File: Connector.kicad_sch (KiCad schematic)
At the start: 5 parts, among them J6 Conn_02x10_Odd_Even

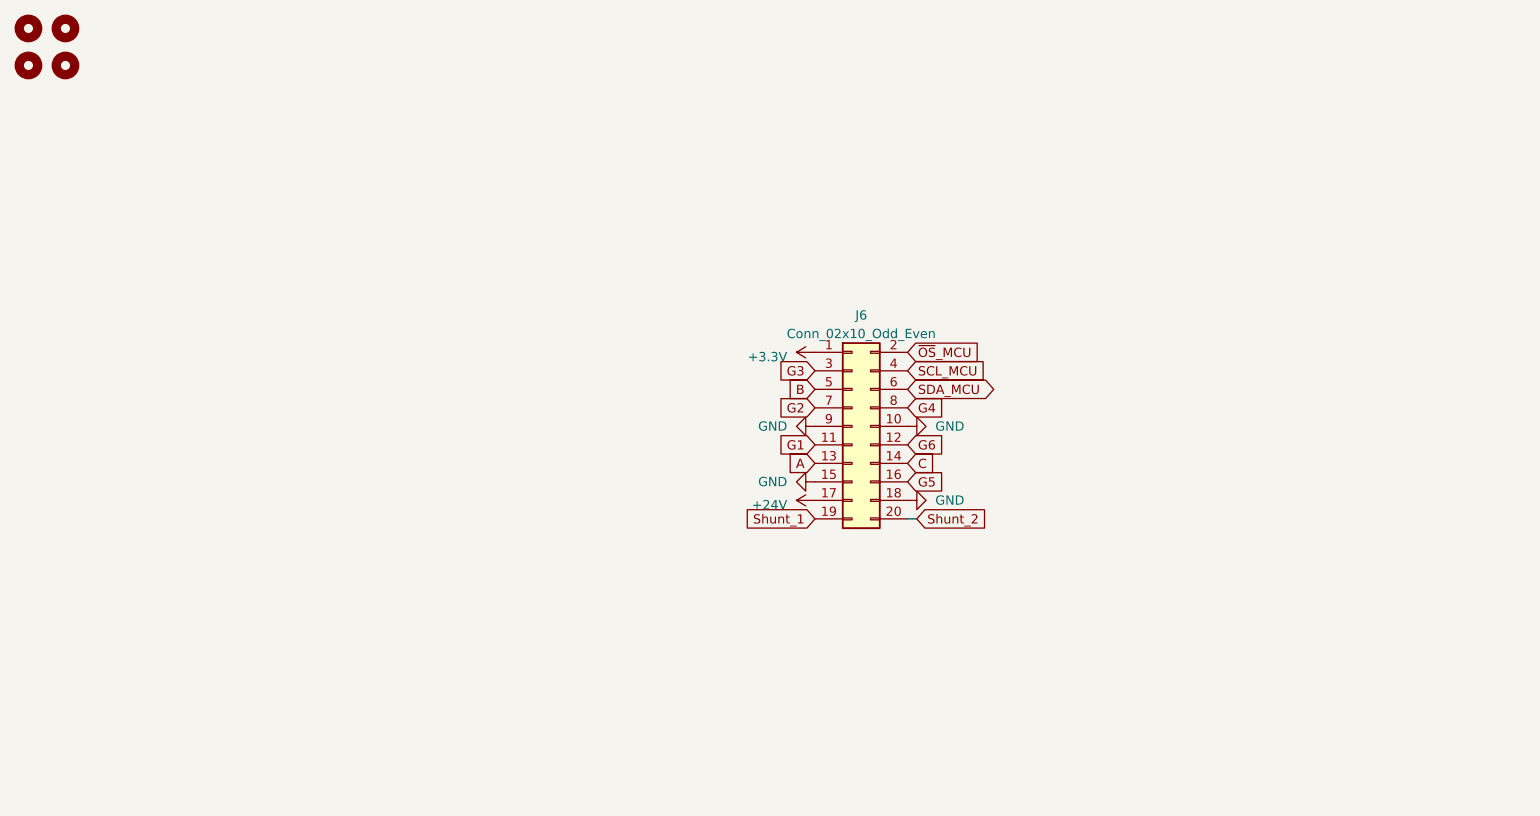
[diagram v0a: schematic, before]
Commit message: Отчётная версия
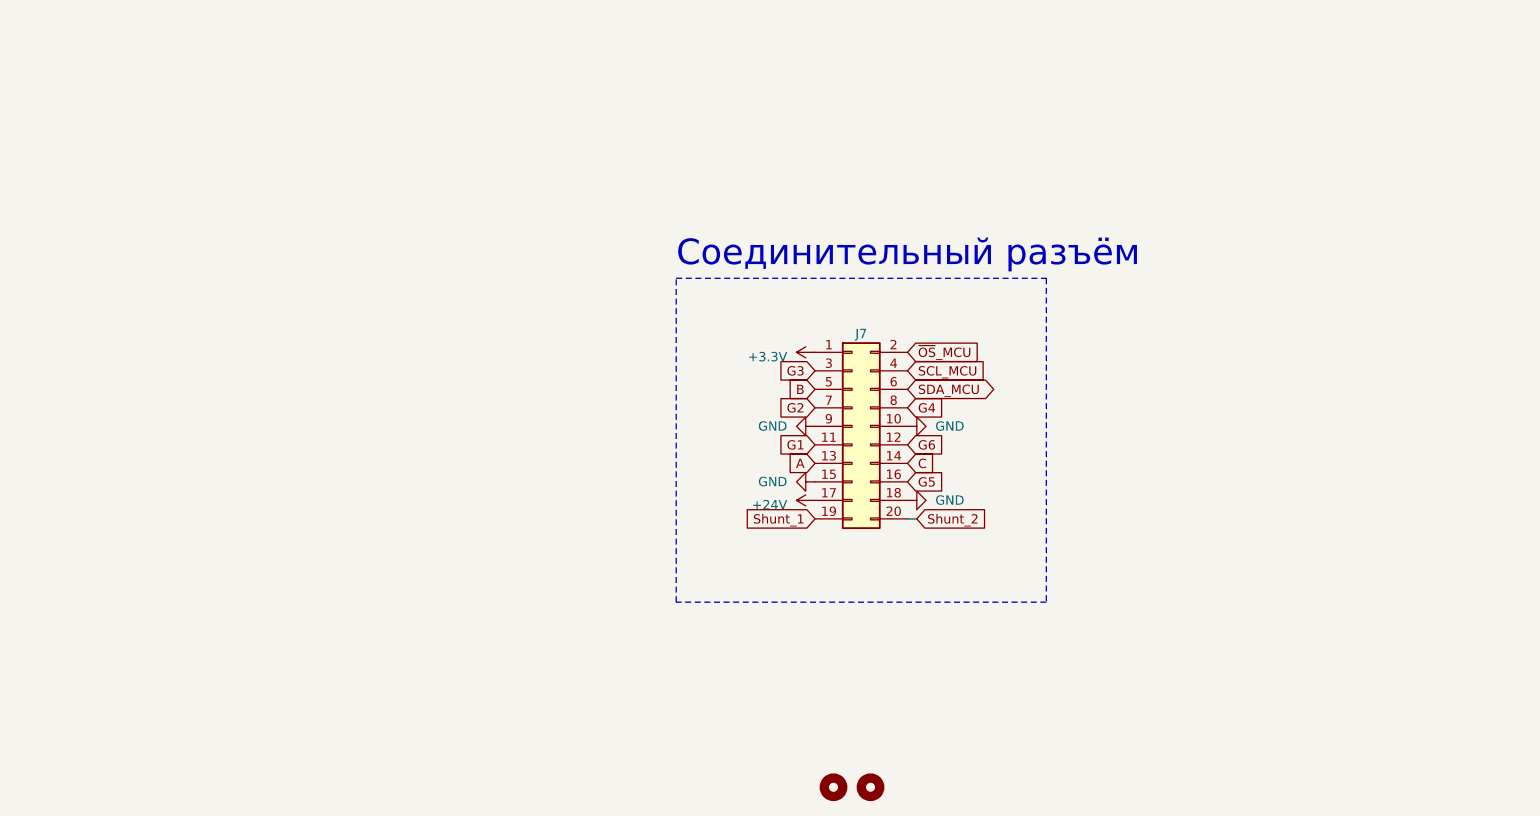
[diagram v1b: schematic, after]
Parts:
- removed H3, H4: MountingHole, MountingHole:MountingHole_3.2mm_M3, symbol Mechanical:MountingHole
- renumbered J6 to J7
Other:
- note added: "Соединительный разъём"
- company: (none) -> Московский Политех
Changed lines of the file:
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@@
 (kicad_sch (version 20230121) (generator eeschema)
   (paper "A4")
+  (title_block
+    (company "Московский Политех")
+    (comment 1 "МПСТ.76721.758764.01.Э3.М")
+  )
   (wire (pts (xy 163.83 96.52) (xy 165.1 96.52))
     (stroke (width 0) (type default))
   )
+  (rectangle (start 132.08 63.5) (end 182.88 107.95)
+    (stroke (width 0) (type dash))
+    (fill (type none))
+  )
+  (text "Соединительный разъём" (at 132.08 62.23 0)
+    (effects (font (size 3.5 3.5)) (justify left bottom))
+  )
   (global_label "C" (shape input) (at 163.83 88.9 0) (fields_autoplaced)
     (effects (font (size 1.27 1.27)) (justify left))
@@
   (symbol (lib_id "power:GND") (at 151.13 91.44 270) (unit 1)
     (in_bom yes) (on_board yes) (dnp no) (fields_autoplaced)
-    (property "Reference" "#PWR018" (at 144.78 91.44 0)
+    (property "Reference" "#PWR019" (at 144.78 91.44 0)
       (effects (font (size 1.27 1.27)) hide)
     )
@@
       (project "Силовая плата"
         (path "/96c6fc92-8ec6-44f7-b0dc-9ad8f1acea09/a27b443f-c036-4fd6-934c-6ea912709de0"
-          (reference "#PWR018") (unit 1)
+          (reference "#PWR019") (unit 1)
+        )
+        (path "/96c6fc92-8ec6-44f7-b0dc-9ad8f1acea09/e8223907-1cc2-45fb-8266-c61760002ef3"
+          (reference "#PWR038") (unit 1)
         )
       )
@@
   )
   (symbol (lib_id "Connector_Generic:Conn_02x10_Odd_Even") (at 156.21 83.82 0) (unit 1)
-    (in_bom yes) (on_board yes) (dnp no) (fields_autoplaced)
-    (property "Reference" "J6" (at 157.48 68.58 0)
+    (in_bom yes) (on_board yes) (dnp no)
+    (property "Reference" "J7" (at 157.48 71.12 0)
       (effects (font (size 1.27 1.27)))
     )
     (property "Value" "Conn_02x10_Odd_Even" (at 157.48 71.12 0)
-      (effects (font (size 1.27 1.27)))
+      (effects (font (size 1.27 1.27)) hide)
     )
     (property "Footprint" "Connector_PinSocket_2.54mm:PinSocket_2x10_P2.54mm_Vertical" (at 156.21 83.82 0)
@@
       (project "Силовая плата"
         (path "/96c6fc92-8ec6-44f7-b0dc-9ad8f1acea09/a27b443f-c036-4fd6-934c-6ea912709de0"
-          (reference "J6") (unit 1)
-        )
-      )
-    )
-  )
-  (symbol (lib_id "Mechanical:MountingHole") (at 48.26 34.29 0) (unit 1)
-    (in_bom yes) (on_board yes) (dnp no) (fields_autoplaced)
-    (property "Reference" "H4" (at 50.8 33.655 0)
-      (effects (font (size 1.27 1.27)) (justify left) hide)
-    )
-    (property "Value" "MountingHole" (at 50.8 36.195 0)
-      (effects (font (size 1.27 1.27)) (justify left) hide)
-    )
-    (property "Footprint" "MountingHole:MountingHole_3.2mm_M3" (at 48.26 34.29 0)
-      (effects (font (size 1.27 1.27)) hide)
-    )
-    (property "Datasheet" "~" (at 48.26 34.29 0)
-      (effects (font (size 1.27 1.27)) hide)
-    )
-    (instances
-      (project "Силовая плата"
-        (path "/96c6fc92-8ec6-44f7-b0dc-9ad8f1acea09/a27b443f-c036-4fd6-934c-6ea912709de0"
-          (reference "H4") (unit 1)
-        )
-      )
-    )
-  )
-  (symbol (lib_id "Mechanical:MountingHole") (at 43.18 34.29 0) (unit 1)
-    (in_bom yes) (on_board yes) (dnp no) (fields_autoplaced)
-    (property "Reference" "H3" (at 45.72 33.655 0)
-      (effects (font (size 1.27 1.27)) (justify left) hide)
-    )
-    (property "Value" "MountingHole" (at 45.72 36.195 0)
-      (effects (font (size 1.27 1.27)) (justify left) hide)
-    )
-    (property "Footprint" "MountingHole:MountingHole_3.2mm_M3" (at 43.18 34.29 0)
-      (effects (font (size 1.27 1.27)) hide)
-    )
-    (property "Datasheet" "~" (at 43.18 34.29 0)
-      (effects (font (size 1.27 1.27)) hide)
-    )
-    (instances
-      (project "Силовая плата"
-        (path "/96c6fc92-8ec6-44f7-b0dc-9ad8f1acea09/a27b443f-c036-4fd6-934c-6ea912709de0"
-          (reference "H3") (unit 1)
+          (reference "J7") (unit 1)
+        )
+        (path "/96c6fc92-8ec6-44f7-b0dc-9ad8f1acea09/e8223907-1cc2-45fb-8266-c61760002ef3"
+          (reference "J9") (unit 1)
         )
       )
@@
         )
         (path "/96c6fc92-8ec6-44f7-b0dc-9ad8f1acea09/a27b443f-c036-4fd6-934c-6ea912709de0"
-          (reference "#PWR023") (unit 1)
+          (reference "#PWR020") (unit 1)
+        )
+        (path "/96c6fc92-8ec6-44f7-b0dc-9ad8f1acea09/e8223907-1cc2-45fb-8266-c61760002ef3"
+          (reference "#PWR039") (unit 1)
         )
       )
@@
   (symbol (lib_id "power:+3.3V") (at 151.13 73.66 90) (unit 1)
     (in_bom yes) (on_board yes) (dnp no) (fields_autoplaced)
-    (property "Reference" "#PWR042" (at 154.94 73.66 0)
+    (property "Reference" "#PWR016" (at 154.94 73.66 0)
       (effects (font (size 1.27 1.27)) hide)
     )
@@
       (project "Силовая плата"
         (path "/96c6fc92-8ec6-44f7-b0dc-9ad8f1acea09/a27b443f-c036-4fd6-934c-6ea912709de0"
-          (reference "#PWR042") (unit 1)
-        )
-      )
-    )
-  )
-  (symbol (lib_id "Mechanical:MountingHole") (at 48.26 29.21 0) (unit 1)
-    (in_bom yes) (on_board yes) (dnp no) (fields_autoplaced)
-    (property "Reference" "H2" (at 50.8 28.575 0)
-      (effects (font (size 1.27 1.27)) (justify left) hide)
-    )
-    (property "Value" "MountingHole" (at 50.8 31.115 0)
-      (effects (font (size 1.27 1.27)) (justify left) hide)
-    )
-    (property "Footprint" "MountingHole:MountingHole_3.2mm_M3" (at 48.26 29.21 0)
-      (effects (font (size 1.27 1.27)) hide)
-    )
-    (property "Datasheet" "~" (at 48.26 29.21 0)
+          (reference "#PWR016") (unit 1)
+        )
+        (path "/96c6fc92-8ec6-44f7-b0dc-9ad8f1acea09/e8223907-1cc2-45fb-8266-c61760002ef3"
+          (reference "#PWR035") (unit 1)
+        )
+      )
+    )
+  )
+  (symbol (lib_id "Mechanical:MountingHole") (at 158.75 133.35 0) (unit 1)
+    (in_bom yes) (on_board yes) (dnp no) (fields_autoplaced)
+    (property "Reference" "H2" (at 161.29 132.715 0)
+      (effects (font (size 1.27 1.27)) (justify left) hide)
+    )
+    (property "Value" "MountingHole" (at 161.29 135.255 0)
+      (effects (font (size 1.27 1.27)) (justify left) hide)
+    )
+    (property "Footprint" "MountingHole:MountingHole_3.2mm_M3" (at 158.75 133.35 0)
+      (effects (font (size 1.27 1.27)) hide)
+    )
+    (property "Datasheet" "~" (at 158.75 133.35 0)
       (effects (font (size 1.27 1.27)) hide)
     )
@@
         (path "/96c6fc92-8ec6-44f7-b0dc-9ad8f1acea09/a27b443f-c036-4fd6-934c-6ea912709de0"
           (reference "H2") (unit 1)
+        )
+        (path "/96c6fc92-8ec6-44f7-b0dc-9ad8f1acea09/e8223907-1cc2-45fb-8266-c61760002ef3"
+          (reference "H4") (unit 1)
         )
       )
@@
           (reference "#PWR017") (unit 1)
         )
-      )
-    )
-  )
-  (symbol (lib_id "Mechanical:MountingHole") (at 43.18 29.21 0) (unit 1)
-    (in_bom yes) (on_board yes) (dnp no) (fields_autoplaced)
-    (property "Reference" "H1" (at 45.72 28.575 0)
-      (effects (font (size 1.27 1.27)) (justify left) hide)
-    )
-    (property "Value" "MountingHole" (at 45.72 31.115 0)
-      (effects (font (size 1.27 1.27)) (justify left) hide)
-    )
-    (property "Footprint" "MountingHole:MountingHole_3.2mm_M3" (at 43.18 29.21 0)
-      (effects (font (size 1.27 1.27)) hide)
-    )
-    (property "Datasheet" "~" (at 43.18 29.21 0)
+        (path "/96c6fc92-8ec6-44f7-b0dc-9ad8f1acea09/e8223907-1cc2-45fb-8266-c61760002ef3"
+          (reference "#PWR036") (unit 1)
+        )
+      )
+    )
+  )
+  (symbol (lib_id "Mechanical:MountingHole") (at 153.67 133.35 0) (unit 1)
+    (in_bom yes) (on_board yes) (dnp no) (fields_autoplaced)
+    (property "Reference" "H1" (at 156.21 132.715 0)
+      (effects (font (size 1.27 1.27)) (justify left) hide)
+    )
+    (property "Value" "MountingHole" (at 156.21 135.255 0)
+      (effects (font (size 1.27 1.27)) (justify left) hide)
+    )
+    (property "Footprint" "MountingHole:MountingHole_3.2mm_M3" (at 153.67 133.35 0)
+      (effects (font (size 1.27 1.27)) hide)
+    )
+    (property "Datasheet" "~" (at 153.67 133.35 0)
       (effects (font (size 1.27 1.27)) hide)
     )
@@
           (reference "H1") (unit 1)
         )
+        (path "/96c6fc92-8ec6-44f7-b0dc-9ad8f1acea09/e8223907-1cc2-45fb-8266-c61760002ef3"
+          (reference "H3") (unit 1)
+        )
       )
     )
@@
   (symbol (lib_id "power:GND") (at 163.83 83.82 90) (mirror x) (unit 1)
     (in_bom yes) (on_board yes) (dnp no) (fields_autoplaced)
-    (property "Reference" "#PWR019" (at 170.18 83.82 0)
+    (property "Reference" "#PWR018" (at 170.18 83.82 0)
       (effects (font (size 1.27 1.27)) hide)
     )
@@
       (project "Силовая плата"
         (path "/96c6fc92-8ec6-44f7-b0dc-9ad8f1acea09/a27b443f-c036-4fd6-934c-6ea912709de0"
-          (reference "#PWR019") (unit 1)
+          (reference "#PWR018") (unit 1)
+        )
+        (path "/96c6fc92-8ec6-44f7-b0dc-9ad8f1acea09/e8223907-1cc2-45fb-8266-c61760002ef3"
+          (reference "#PWR037") (unit 1)
         )
       )
@@
   (symbol (lib_id "power:GND") (at 163.83 93.98 90) (mirror x) (unit 1)
     (in_bom yes) (on_board yes) (dnp no) (fields_autoplaced)
-    (property "Reference" "#PWR022" (at 170.18 93.98 0)
+    (property "Reference" "#PWR021" (at 170.18 93.98 0)
       (effects (font (size 1.27 1.27)) hide)
     )
@@
       (project "Силовая плата"
         (path "/96c6fc92-8ec6-44f7-b0dc-9ad8f1acea09/a27b443f-c036-4fd6-934c-6ea912709de0"
-          (reference "#PWR022") (unit 1)
-        )
-      )
+          (reference "#PWR021") (unit 1)
+        )
+        (path "/96c6fc92-8ec6-44f7-b0dc-9ad8f1acea09/e8223907-1cc2-45fb-8266-c61760002ef3"
+          (reference "#PWR040") (unit 1)
+        )
+      )
